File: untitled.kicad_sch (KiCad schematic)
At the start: 4 parts, among them J1 USB_B_Micro, J2 Conn_01x04_Pin, J3 Conn_01x14_Pin

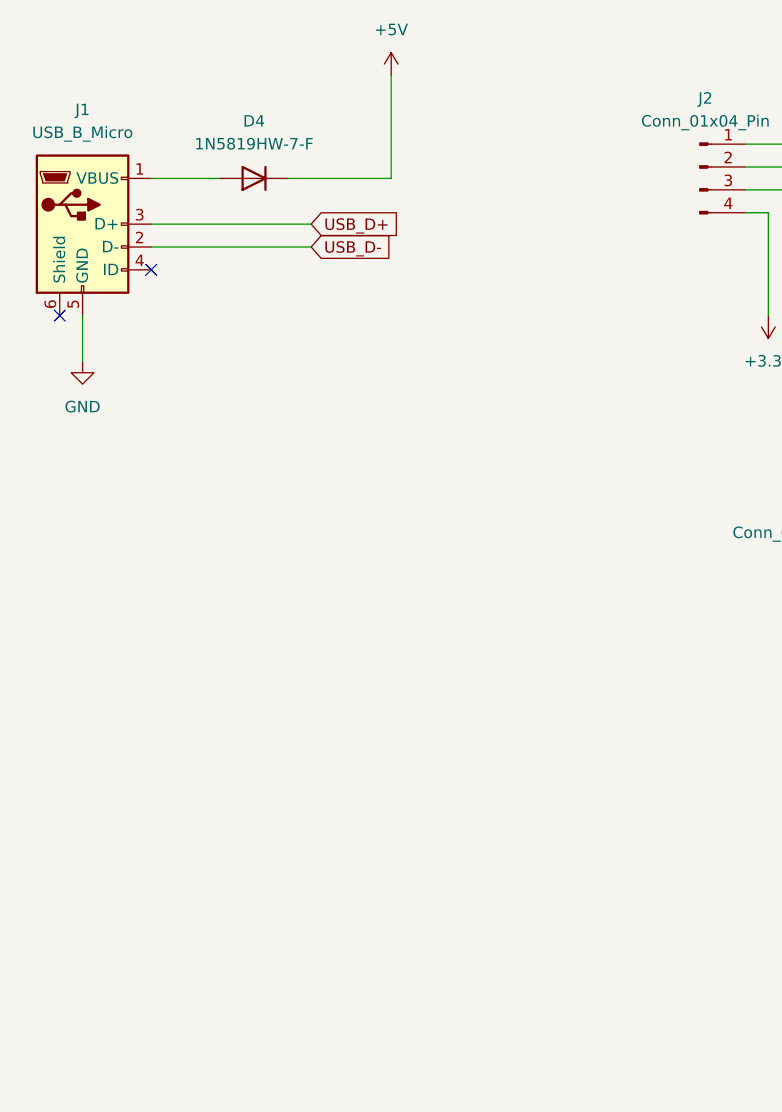
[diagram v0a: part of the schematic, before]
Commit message: Update to V2.1
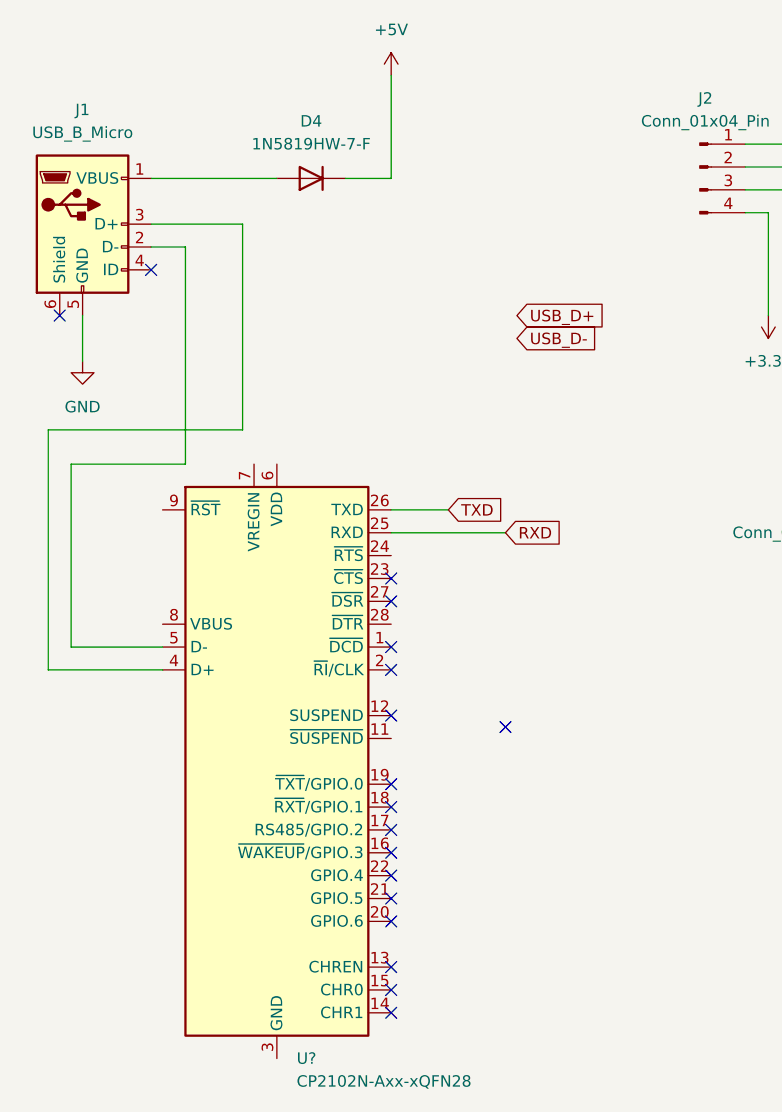
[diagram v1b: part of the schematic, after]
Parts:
- added U?: CP2102N-Axx-xQFN28, Package_DFN_QFN:QFN-28-1EP_5x5mm_P0.5mm_EP3.35x3.35mm, symbol Interface_USB:CP2102N-Axx-xQFN28
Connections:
- net USB_D+: no longer J1.3 (D+)
- net USB_D-: no longer J1.2 (D-)
- new net: U?.29 (GND), U?.3 (GND)
- new net: J1.3 (D+), U?.4 (D+)
- new net: J1.2 (D-), U?.5 (D-)
- new net RXD: U?.25 (RXD)
- new net TXD: U?.26 (TXD)
- no-connect marks 2 -> 18
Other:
- moved on the sheet: D4
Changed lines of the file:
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@@
 (kicad_sch (version 20230121) (generator eeschema)
   (paper "A4")
+  (no_connect (at 74.93 93.98))
+  (no_connect (at 87.63 95.25))
+  (no_connect (at 74.93 106.68))
+  (no_connect (at 74.93 114.3))
+  (no_connect (at 74.93 104.14))
   (no_connect (at 38.1 49.53))
+  (no_connect (at 74.93 116.84))
+  (no_connect (at 74.93 124.46))
+  (no_connect (at 74.93 81.28))
+  (no_connect (at 74.93 109.22))
+  (no_connect (at 74.93 111.76))
+  (no_connect (at 74.93 121.92))
+  (no_connect (at 74.93 88.9))
+  (no_connect (at 74.93 86.36))
+  (no_connect (at 74.93 101.6))
   (no_connect (at 48.26 44.45))
+  (no_connect (at 74.93 127))
+  (no_connect (at 74.93 78.74))
   (wire (pts (xy 124.46 88.9) (xy 147.32 88.9))
     (stroke (width 0) (type default))
@@
     (stroke (width 0) (type default))
   )
+  (wire (pts (xy 58.42 62.23) (xy 36.83 62.23))
+    (stroke (width 0) (type default))
+  )
+  (wire (pts (xy 48.26 41.91) (xy 52.07 41.91))
+    (stroke (width 0) (type default))
+  )
   (wire (pts (xy 142.24 109.22) (xy 124.46 109.22))
     (stroke (width 0) (type default))
   )
-  (wire (pts (xy 63.5 34.29) (xy 74.93 34.29))
+  (wire (pts (xy 69.85 34.29) (xy 74.93 34.29))
     (stroke (width 0) (type default))
   )
@@
     (stroke (width 0) (type default))
   )
+  (wire (pts (xy 52.07 41.91) (xy 52.07 66.04))
+    (stroke (width 0) (type default))
+  )
   (wire (pts (xy 142.24 116.84) (xy 142.24 109.22))
     (stroke (width 0) (type default))
@@
     (stroke (width 0) (type default))
   )
+  (wire (pts (xy 74.93 71.12) (xy 81.28 71.12))
+    (stroke (width 0) (type default))
+  )
   (wire (pts (xy 124.46 35.56) (xy 124.46 36.83))
     (stroke (width 0) (type default))
   )
+  (wire (pts (xy 36.83 88.9) (xy 49.53 88.9))
+    (stroke (width 0) (type default))
+  )
+  (wire (pts (xy 39.37 86.36) (xy 49.53 86.36))
+    (stroke (width 0) (type default))
+  )
   (wire (pts (xy 158.75 109.22) (xy 144.78 109.22))
     (stroke (width 0) (type default))
@@
     (stroke (width 0) (type default))
   )
-  (wire (pts (xy 48.26 34.29) (xy 55.88 34.29))
+  (wire (pts (xy 48.26 34.29) (xy 62.23 34.29))
     (stroke (width 0) (type default))
   )
@@
     (stroke (width 0) (type default))
   )
+  (wire (pts (xy 36.83 62.23) (xy 36.83 88.9))
+    (stroke (width 0) (type default))
+  )
   (wire (pts (xy 158.75 113.03) (xy 143.51 113.03))
     (stroke (width 0) (type default))
@@
     (stroke (width 0) (type default))
   )
-  (wire (pts (xy 48.26 39.37) (xy 66.04 39.37))
-    (stroke (width 0) (type default))
-  )
   (wire (pts (xy 144.78 83.82) (xy 144.78 78.74))
     (stroke (width 0) (type default))
   )
+  (wire (pts (xy 48.26 39.37) (xy 58.42 39.37))
+    (stroke (width 0) (type default))
+  )
   (wire (pts (xy 147.32 96.52) (xy 124.46 96.52))
     (stroke (width 0) (type default))
@@
     (stroke (width 0) (type default))
   )
+  (wire (pts (xy 39.37 66.04) (xy 39.37 86.36))
+    (stroke (width 0) (type default))
+  )
   (wire (pts (xy 124.46 99.06) (xy 147.32 99.06))
     (stroke (width 0) (type default))
@@
     (stroke (width 0) (type default))
   )
-  (wire (pts (xy 48.26 41.91) (xy 66.04 41.91))
-    (stroke (width 0) (type default))
-  )
   (wire (pts (xy 134.62 78.74) (xy 124.46 78.74))
     (stroke (width 0) (type default))
@@
     (stroke (width 0) (type default))
   )
+  (wire (pts (xy 52.07 66.04) (xy 39.37 66.04))
+    (stroke (width 0) (type default))
+  )
+  (wire (pts (xy 58.42 39.37) (xy 58.42 62.23))
+    (stroke (width 0) (type default))
+  )
   (wire (pts (xy 158.75 97.79) (xy 147.32 97.79))
     (stroke (width 0) (type default))
@@
     (stroke (width 0) (type default))
   )
+  (wire (pts (xy 74.93 73.66) (xy 87.63 73.66))
+    (stroke (width 0) (type default))
+  )
   (global_label "U-TX" (shape input) (at 128.27 36.83 0) (fields_autoplaced)
     (effects (font (size 1.27 1.27)) (justify left))
@@
     )
   )
+  (global_label "RXD" (shape input) (at 87.63 73.66 0) (fields_autoplaced)
+    (effects (font (size 1.27 1.27)) (justify left))
+    (property "Intersheetrefs" "${INTERSHEET_REFS}" (at 94.3647 73.66 0)
+      (effects (font (size 1.27 1.27)) (justify left) hide)
+    )
+  )
   (global_label "IO6" (shape input) (at 158.75 101.6 0) (fields_autoplaced)
     (effects (font (size 1.27 1.27)) (justify left))
@@
     )
   )
+  (global_label "TXD" (shape input) (at 81.28 71.12 0) (fields_autoplaced)
+    (effects (font (size 1.27 1.27)) (justify left))
+    (property "Intersheetrefs" "${INTERSHEET_REFS}" (at 87.7123 71.12 0)
+      (effects (font (size 1.27 1.27)) (justify left) hide)
+    )
+  )
   (global_label "IO0" (shape input) (at 158.75 78.74 0) (fields_autoplaced)
     (effects (font (size 1.27 1.27)) (justify left))
@@
     )
   )
-  (global_label "USB_D+" (shape input) (at 66.04 39.37 0) (fields_autoplaced)
-    (effects (font (size 1.27 1.27)) (justify left))
-    (property "Intersheetrefs" "${INTERSHEET_REFS}" (at 76.6452 39.37 0)
-      (effects (font (size 1.27 1.27)) (justify left) hide)
-    )
-  )
-  (global_label "USB_D-" (shape input) (at 66.04 41.91 0) (fields_autoplaced)
-    (effects (font (size 1.27 1.27)) (justify left))
-    (property "Intersheetrefs" "${INTERSHEET_REFS}" (at 76.6452 41.91 0)
+  (global_label "USB_D+" (shape input) (at 88.9 49.53 0) (fields_autoplaced)
+    (effects (font (size 1.27 1.27)) (justify left))
+    (property "Intersheetrefs" "${INTERSHEET_REFS}" (at 99.5052 49.53 0)
+      (effects (font (size 1.27 1.27)) (justify left) hide)
+    )
+  )
+  (global_label "USB_D-" (shape input) (at 88.9 52.07 0) (fields_autoplaced)
+    (effects (font (size 1.27 1.27)) (justify left))
+    (property "Intersheetrefs" "${INTERSHEET_REFS}" (at 99.5052 52.07 0)
       (effects (font (size 1.27 1.27)) (justify left) hide)
     )
@@
         (path "/9ef41b73-8dcb-4021-8930-5b1db22eb182/1969c3e8-6100-4b45-a4c4-adbf98ab0c9d"
           (reference "#PWR07") (unit 1)
+        )
+      )
+    )
+  )
+  (symbol (lib_id "Interface_USB:CP2102N-Axx-xQFN28") (at 62.23 99.06 0) (unit 1)
+    (in_bom yes) (on_board yes) (dnp no) (fields_autoplaced)
+    (property "Reference" "U?" (at 64.4241 132.08 0)
+      (effects (font (size 1.27 1.27)) (justify left))
+    )
+    (property "Value" "CP2102N-Axx-xQFN28" (at 64.4241 134.62 0)
+      (effects (font (size 1.27 1.27)) (justify left))
+    )
+    (property "Footprint" "Package_DFN_QFN:QFN-28-1EP_5x5mm_P0.5mm_EP3.35x3.35mm" (at 95.25 130.81 0)
+      (effects (font (size 1.27 1.27)) hide)
+    )
+    (property "Datasheet" "https://www.silabs.com/documents/public/data-sheets/cp2102n-datasheet.pdf" (at 63.5 118.11 0)
+      (effects (font (size 1.27 1.27)) hide)
+    )
+    (pin "14")
+    (pin "10")
+    (pin "11")
+    (pin "17")
+    (pin "1")
+    (pin "16")
+    (pin "18")
+    (pin "15")
+    (pin "13")
+    (pin "9")
+    (pin "8")
+    (pin "7")
+    (pin "6")
+    (pin "5")
+    (pin "4")
+    (pin "3")
+    (pin "29")
+    (pin "28")
+    (pin "27")
+    (pin "26")
+    (pin "25")
+    (pin "24")
+    (pin "23")
+    (pin "22")
+    (pin "21")
+    (pin "20")
+    (pin "2")
+    (pin "19")
+    (pin "12")
+    (instances
+      (project "Julelys V2"
+        (path "/9ef41b73-8dcb-4021-8930-5b1db22eb182/75d2635a-f2eb-4079-86f3-082e38564c79"
+          (reference "U?") (unit 1)
+        )
+        (path "/9ef41b73-8dcb-4021-8930-5b1db22eb182/1969c3e8-6100-4b45-a4c4-adbf98ab0c9d"
+          (reference "U?") (unit 1)
         )
       )
@@
     )
   )
-  (symbol (lib_id "Device:D") (at 59.69 34.29 180) (unit 1)
-    (in_bom yes) (on_board yes) (dnp no) (fields_autoplaced)
-    (property "Reference" "D4" (at 59.69 27.94 0)
-      (effects (font (size 1.27 1.27)))
-    )
-    (property "Value" "1N5819HW-7-F" (at 59.69 30.48 0)
-      (effects (font (size 1.27 1.27)))
-    )
-    (property "Footprint" "Diode_SMD:D_SOD-123" (at 59.69 34.29 0)
-      (effects (font (size 1.27 1.27)) hide)
-    )
-    (property "Datasheet" "~" (at 59.69 34.29 0)
-      (effects (font (size 1.27 1.27)) hide)
-    )
-    (property "Sim.Device" "D" (at 59.69 34.29 0)
-      (effects (font (size 1.27 1.27)) hide)
-    )
-    (property "Sim.Pins" "1=K 2=A" (at 59.69 34.29 0)
-      (effects (font (size 1.27 1.27)) hide)
-    )
+  (symbol (lib_id "Device:D") (at 66.04 34.29 180) (unit 1)
+    (in_bom yes) (on_board yes) (dnp no) (fields_autoplaced)
+    (property "Reference" "D4" (at 66.04 27.94 0)
+      (effects (font (size 1.27 1.27)))
+    )
+    (property "Value" "1N5819HW-7-F" (at 66.04 30.48 0)
+      (effects (font (size 1.27 1.27)))
+    )
+    (property "Footprint" "Diode_SMD:D_SOD-123" (at 66.04 34.29 0)
+      (effects (font (size 1.27 1.27)) hide)
+    )
+    (property "Datasheet" "~" (at 66.04 34.29 0)
+      (effects (font (size 1.27 1.27)) hide)
+    )
+    (property "Sim.Device" "D" (at 66.04 34.29 0)
+      (effects (font (size 1.27 1.27)) hide)
+    )
+    (property "Sim.Pins" "1=K 2=A" (at 66.04 34.29 0)
+      (effects (font (size 1.27 1.27)) hide)
+    )

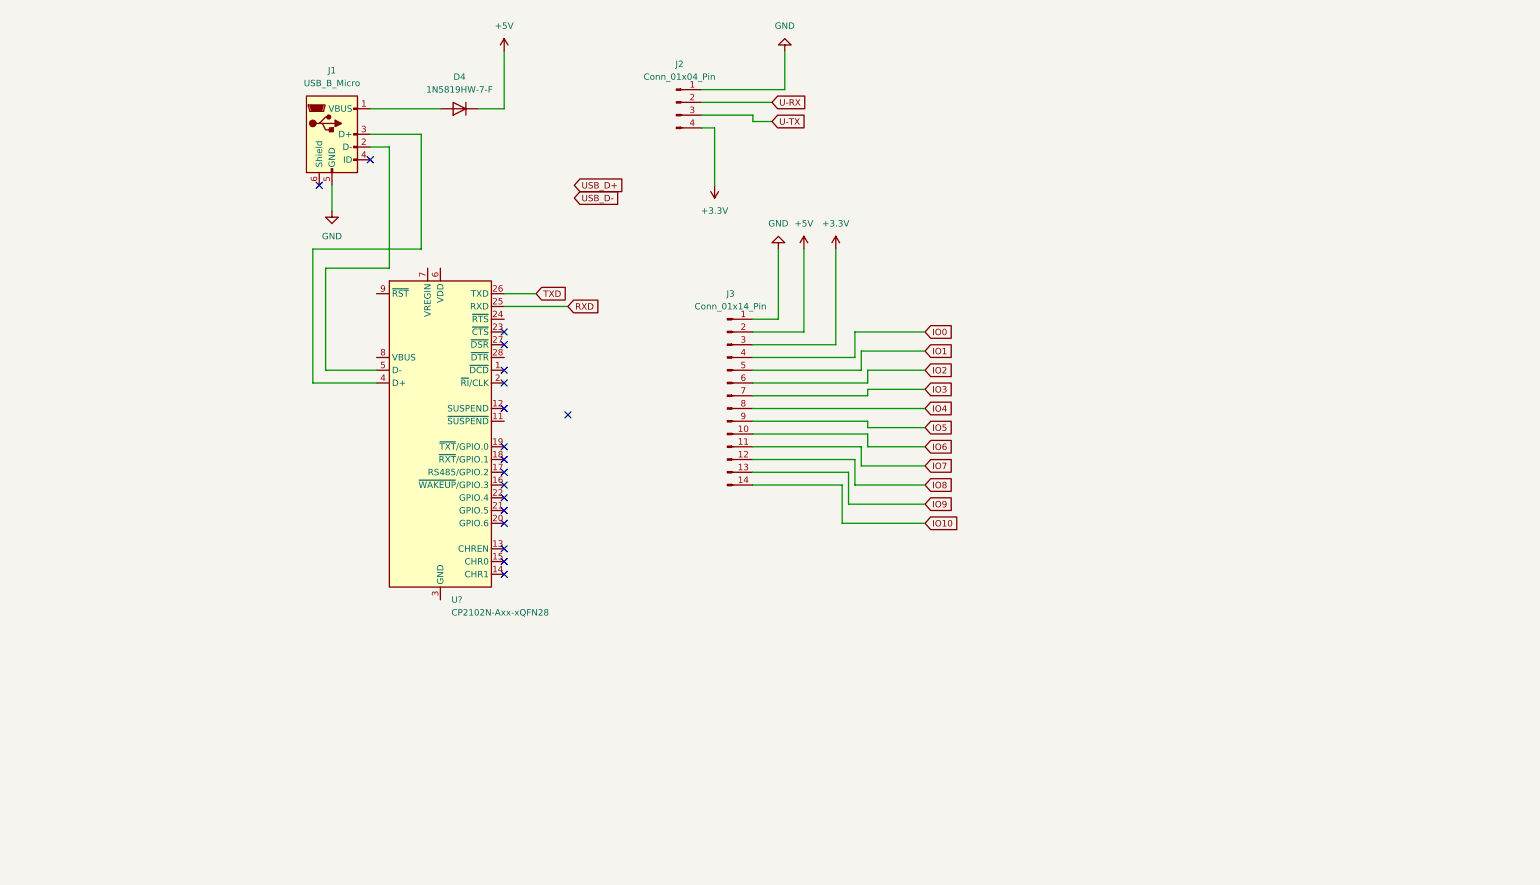
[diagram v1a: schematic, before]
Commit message: version 3
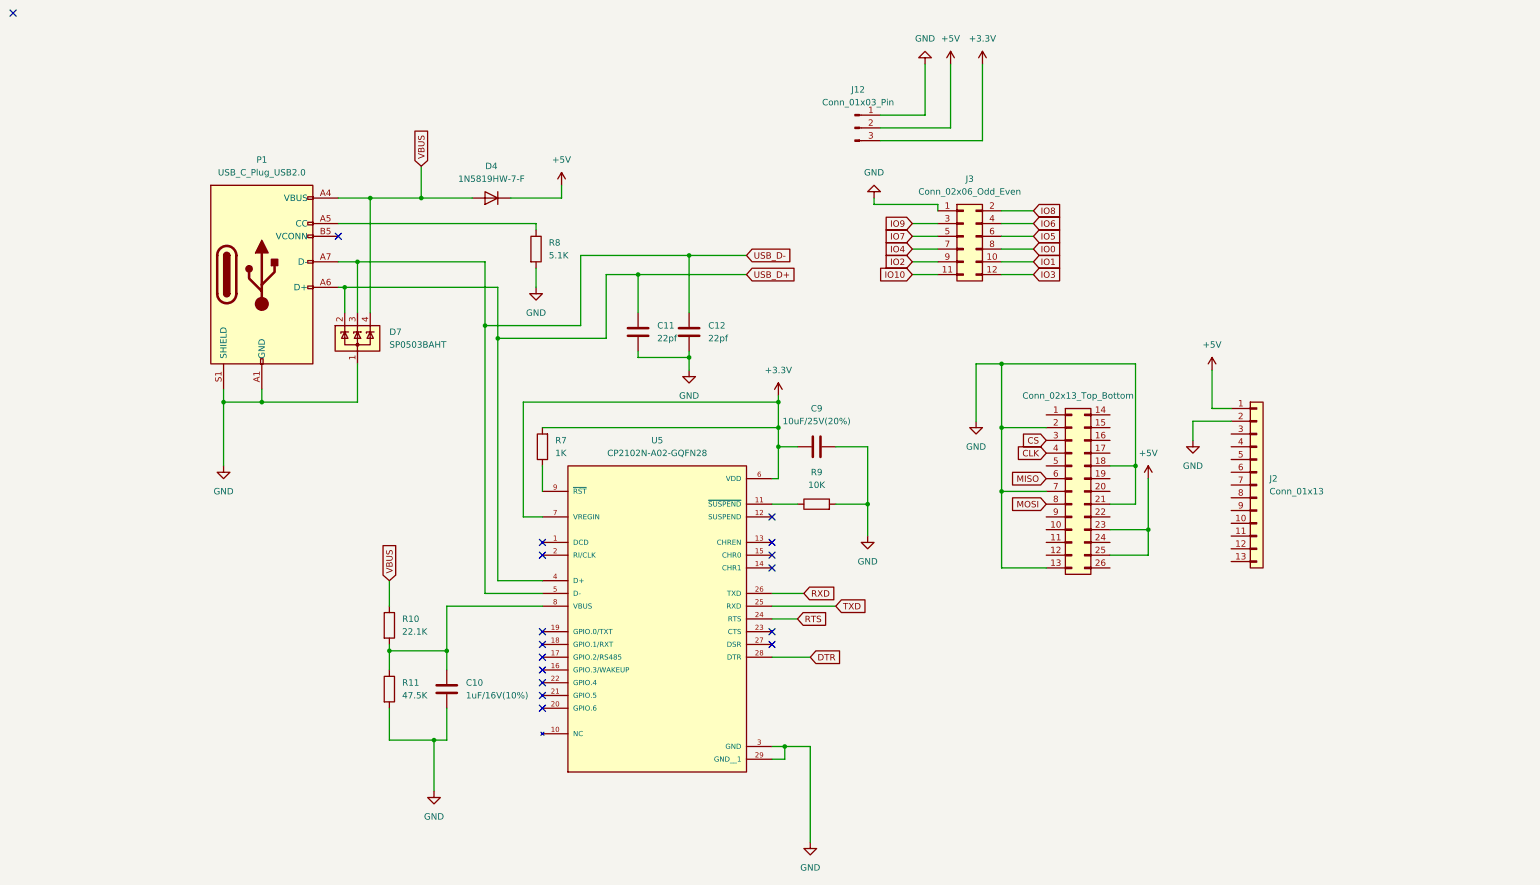
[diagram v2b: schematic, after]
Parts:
- removed J1: USB_B_Micro, X62D-B-5PA8_FOOTPRINT:CONN_ZX62D-B-5PA830_HIR, symbol Connector:USB_B_Micro
- removed J2: Conn_01x04_Pin, Connector_PinHeader_2.54mm:PinHeader_1x04_P2.54mm_Vertical, symbol Connector:Conn_01x04_Pin
- removed J3: Conn_01x14_Pin, Connector_PinHeader_2.54mm:PinHeader_1x14_P2.54mm_Vertical, symbol Connector:Conn_01x14_Pin
- removed U?: CP2102N-Axx-xQFN28, Package_DFN_QFN:QFN-28-1EP_5x5mm_P0.5mm_EP3.35x3.35mm, symbol Interface_USB:CP2102N-Axx-xQFN28
- added C10: 1uF/16V(10%), Capacitor_SMD:C_0402_1005Metric, symbol Device:C
- added C11, C12: 22pf, Capacitor_SMD:C_0603_1608Metric, symbol Device:C
- added C9: 10uF/25V(20%), Capacitor_SMD:C_0402_1005Metric, symbol Device:C
- added D7: SP0503BAHT, Package_TO_SOT_SMD:SOT-143, symbol Power_Protection:SP0503BAHT
- added J1: Conn_02x13_Top_Bottom, Connector_PinSocket_2.54mm:PinSocket_2x13_P2.54mm_Vertical, symbol Connector_Generic:Conn_02x13_Top_Bottom
- added J12: Conn_01x03_Pin, Connector_PinHeader_2.54mm:PinHeader_1x03_P2.54mm_Vertical, symbol Connector:Conn_01x03_Pin
- added J2: Conn_01x13, Connector_PinSocket_2.54mm:PinSocket_1x13_P2.54mm_Vertical, symbol Connector_Generic:Conn_01x13
- added J3: Conn_02x06_Odd_Even, Connector_PinHeader_2.54mm:PinHeader_2x06_P2.54mm_Vertical, symbol Connector_Generic:Conn_02x06_Odd_Even
- added P1: USB_C_Plug_USB2.0, Connector_USB:USB_C_Receptacle_HRO_TYPE-C-31-M-12, symbol Connector:USB_C_Plug_USB2.0
- added R10: 22.1K, Resistor_SMD:R_0402_1005Metric, symbol Device:R
- added R11: 47.5K, Resistor_SMD:R_0402_1005Metric, symbol Device:R
- added R7: 1K, Resistor_SMD:R_0402_1005Metric, symbol Device:R
- added R8: 5.1K, Resistor_SMD:R_0603_1608Metric, symbol Device:R
- added R9: 10K, Resistor_SMD:R_0402_1005Metric, symbol Device:R
- added U5: CP2102N-A02-GQFN28, Connector_USB:QFN50P500X500X80-29N, symbol Interface_USB:CP2102N-A02-GQFN28
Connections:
- net +3.3V: now also C9.1, J12.3 (Pin_3), R7.2, U5.6 (VDD), U5.7 (VREGIN)
- net +5V: now also J1.23 (Pin_23), J1.25 (Pin_25), J12.2 (Pin_2), J2.1 (Pin_1)
- net GND: now also C10.2, C11.2, C12.2, C9.2, D7.1 (A), J1.13 (Pin_13), J1.18 (Pin_18), J1.2 (Pin_2), J1.21 (Pin_21), J1.7 (Pin_7), J12.1 (Pin_1), J2.2 (Pin_2), J3.1 (Pin_1), P1.A1 (GND), P1.A12 (GND), P1.B1 (GND), P1.B12 (GND), P1.S1 (SHIELD), R11.2, R8.2, R9.2, U5.29 (GND__1), U5.3 (GND)
- net IO0: now also J3.8 (Pin_8)
- net IO1: now also J3.10 (Pin_10)
- net IO10: now also J3.11 (Pin_11)
- net IO2: now also J3.9 (Pin_9)
- net IO3: now also J3.12 (Pin_12)
- net IO4: now also J3.7 (Pin_7)
- net IO5: now also J3.6 (Pin_6)
- net IO6: now also J3.4 (Pin_4)
- net IO7: now also J3.5 (Pin_5)
- net IO8: now also J3.2 (Pin_2)
- net IO9: now also J3.3 (Pin_3)
- net RXD: now also U5.26 (TXD)
- net TXD: now also U5.25 (RXD)
- net USB_D+: now also C11.1, D7.2 (K), P1.A6 (D+), U5.4 (D+)
- net USB_D-: now also C12.1, D7.3 (K), P1.A7 (D-), U5.5 (D-)
- net VBUS: now reaches D4.2 (A)
- net VBUS: now also D7.4 (K), P1.A4 (VBUS), P1.A9 (VBUS), P1.B4 (VBUS), P1.B9 (VBUS), R10.1
- new net: R9.1, U5.11 (~{SUSPEND})
- new net: C10.1, R10.2, R11.1, U5.8 (VBUS)
- new net: R7.1, U5.9 (~{RST})
- new net: P1.A5 (CC), R8.1
- new net CLK: J1.4 (Pin_4)
- new net CS: J1.3 (Pin_3)
- new net DTR: U5.28 (DTR)
- new net MISO: J1.6 (Pin_6)
- new net MOSI: J1.8 (Pin_8)
- new net RTS: U5.24 (RTS)
- no-connect marks 18 -> 17
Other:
- moved on the sheet: D4
